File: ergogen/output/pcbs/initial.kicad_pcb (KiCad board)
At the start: 2 copper layers, 190.8 x 90.6 mm, 57 parts

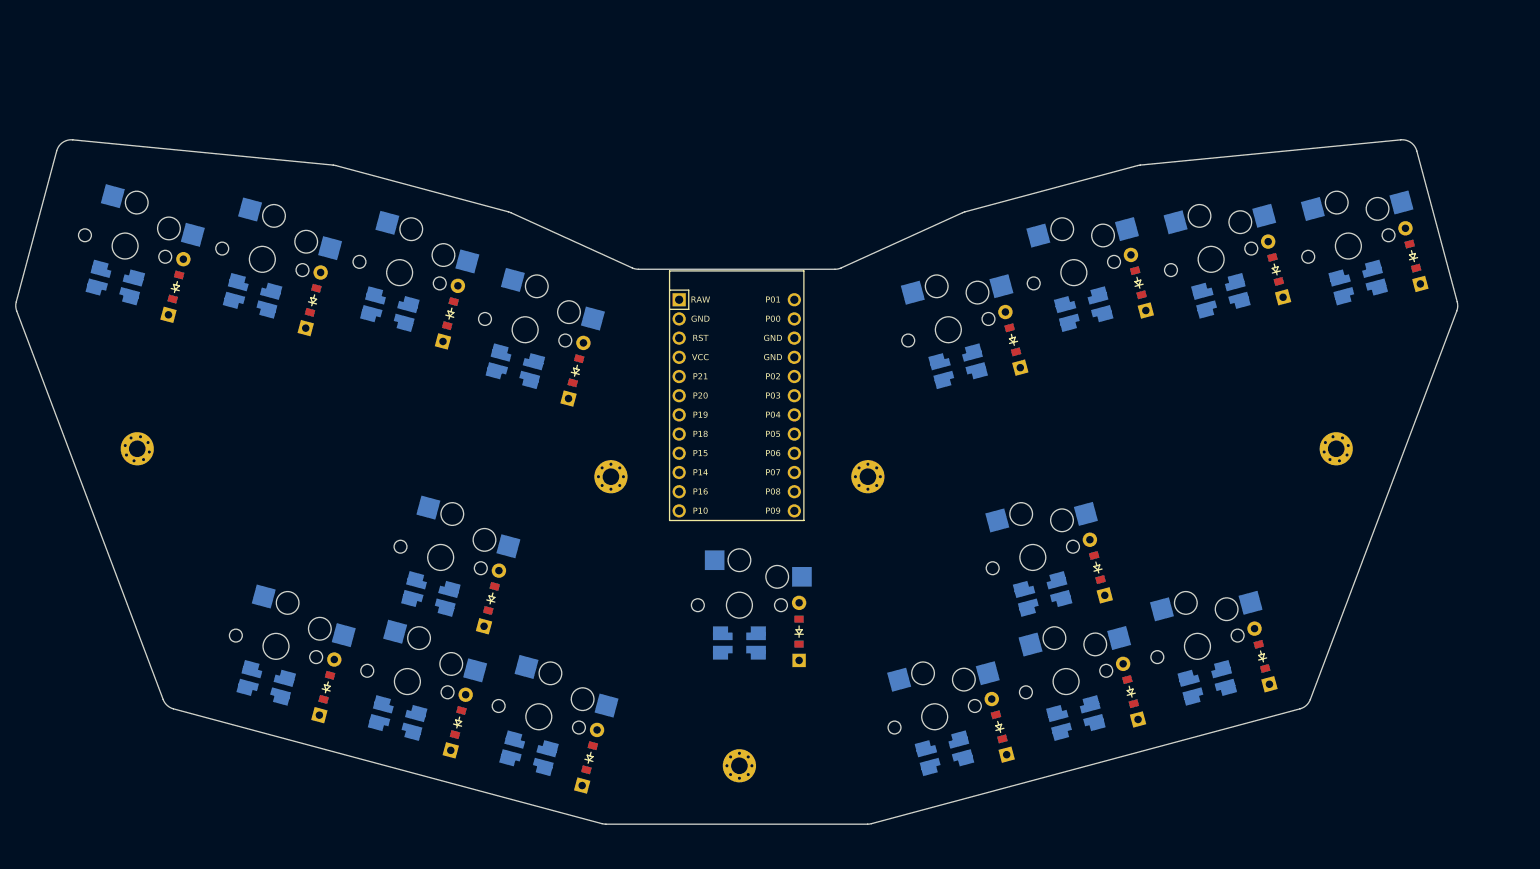
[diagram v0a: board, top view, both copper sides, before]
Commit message: yknow what eight keys
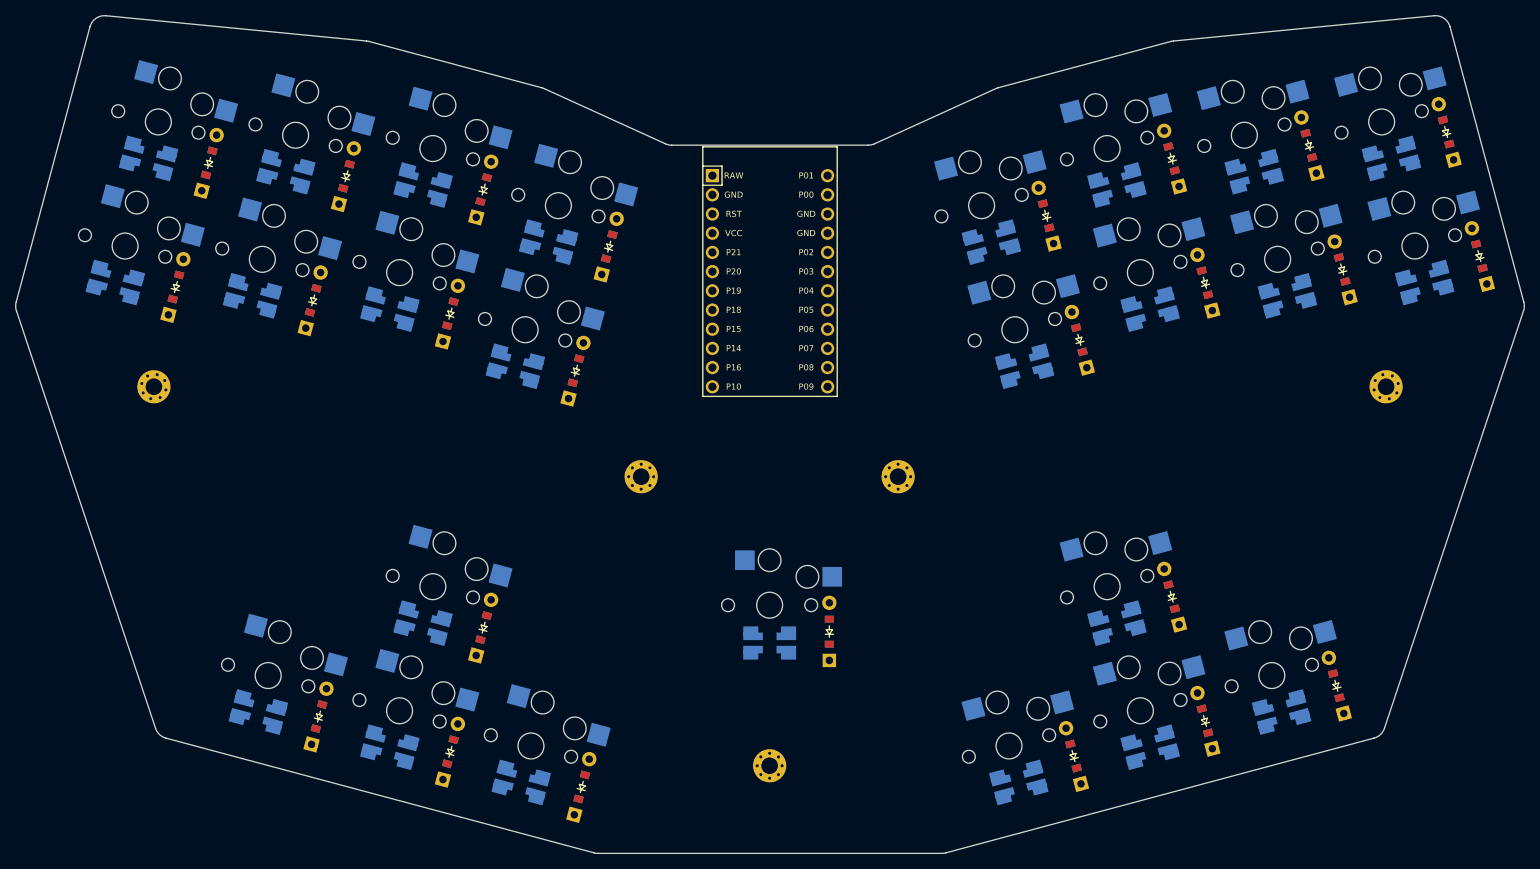
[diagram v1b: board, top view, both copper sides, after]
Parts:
- added D18: , ComboDiode, F.Cu at (213.6, 127.3)
- added D19: , ComboDiode, F.Cu at (209.2, 110.9)
- added D20: , ComboDiode, F.Cu at (197.0, 134.9)
- added D21: , ComboDiode, F.Cu at (192.6, 118.5)
- added D22: , ComboDiode, F.Cu at (231.0, 180.6)
- added D23: , ComboDiode, F.Cu at (213.6, 185.3)
- added D24: , ComboDiode, F.Cu at (209.2, 168.9)
- added D25: , ComboDiode, F.Cu at (196.2, 190.0)
- added LED18: , WS2812B, F.Cu at (206.4, 130.8)
- added LED19: , WS2812B, F.Cu at (202.0, 114.4)
- added LED20: , WS2812B, F.Cu at (189.7, 138.4)
- added LED21: , WS2812B, F.Cu at (185.3, 122.0)
- added LED22: , WS2812B, F.Cu at (223.7, 184.1)
- added LED23: , WS2812B, F.Cu at (206.4, 188.8)
- added LED24: , WS2812B, F.Cu at (202.0, 172.4)
- added LED25: , WS2812B, F.Cu at (189.0, 193.5)
- added S18: , PG1350, F.Cu at (205.1, 126.0)
- added S19: , PG1350, F.Cu at (200.7, 109.6)
- added S20: , PG1350, F.Cu at (188.4, 133.6)
- added S21: , PG1350, F.Cu at (184.0, 117.1)
- added S22: , PG1350, F.Cu at (222.4, 179.3)
- added S23: , PG1350, F.Cu at (205.1, 184.0)
- added S24: , PG1350, F.Cu at (200.7, 167.5)
- added S25: , PG1350, F.Cu at (187.7, 188.6)
- moved D10 143.3 mm to (113.8, 189.4), turned to 75 degrees
- moved LED10 142.1 mm to (105.7, 188.8), turned to -15 degrees
- moved S10 139.8 mm to (107.0, 184.0), turned to -15 degrees
- moved D11 115.0 mm to (118.2, 173.0), turned to 75 degrees
- moved LED11 114.1 mm to (110.1, 172.4), turned to -15 degrees
- moved S11 111.7 mm to (111.4, 167.5), turned to -15 degrees
- moved D12 99.4 mm to (131.1, 194.1), turned to 75 degrees
- moved LED12 97.3 mm to (123.1, 193.5), turned to -15 degrees
- moved S12 95.3 mm to (124.4, 188.6), turned to -15 degrees
- moved D17 87.2 mm to (227.4, 109.2)
- moved S17 87.2 mm to (218.8, 107.8)
- moved LED17 87.2 mm to (220.1, 112.6)
- moved D15 85.0 mm to (245.5, 107.4)
- moved S15 85.0 mm to (237.0, 106.1)
- moved LED15 85.0 mm to (238.3, 110.9)
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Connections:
- net mirror_home_top renamed mirror_ring_bottom
- net mirror_near_thumb renamed mirror_pinky_bottom
- D1 pad 1: P16 -> P19
- D1 pad 2: pinky_home -> pinky_bottom
- D10 pad 1: P6 -> P10
- D10 pad 2: mirror_pinky_home -> home_thumb
- D11 pad 1: P6 -> P8
- D11 pad 2: mirror_ring_home -> home_top
- D12 pad 1: P6 -> P10
- D12 pad 2: mirror_middle_home -> far_thumb
- D13 pad 1: P6 -> P8
- D13 pad 2: mirror_index_home -> main_default
- D14 pad 1: P9 -> P4
- D15 pad 1: P9 -> P6
- D15 pad 2: mirror_home_thumb -> mirror_pinky_home
- D16 pad 1: P8 -> P4
- D17 pad 1: P9 -> P6
- D17 pad 2: mirror_far_thumb -> mirror_ring_home
- D2 pad 2: ring_home -> pinky_home
- D3 pad 1: P16 -> P19
- D3 pad 2: middle_home -> ring_bottom
- D4 pad 2: index_home -> ring_home
- D5 pad 1: P10 -> P19
- D5 pad 2: near_thumb -> middle_bottom
- D6 pad 1: P10 -> P16
- D6 pad 2: home_thumb -> middle_home
- D7 pad 1: P8 -> P19
- D7 pad 2: home_top -> index_bottom
- D8 pad 1: P10 -> P16
- D8 pad 2: far_thumb -> index_home
- D9 pad 1: P8 -> P10
- D9 pad 2: main_default -> near_thumb
- LED1 pad 2: P18 -> P14
- LED1 pad 22: P18 -> P14
- LED1 pad 4: P18 -> P14
- LED1 pad 44: P18 -> P14
- LED10 pad 2: P18 -> P14
- LED10 pad 22: P18 -> P14
- LED10 pad 4: P18 -> P14
- LED10 pad 44: P18 -> P14
- LED11 pad 2: P18 -> P14
- LED11 pad 22: P18 -> P14
- LED11 pad 4: P18 -> P14
- LED11 pad 44: P18 -> P14
- LED12 pad 2: P18 -> P14
- LED12 pad 22: P18 -> P14
- LED12 pad 4: P18 -> P14
- LED12 pad 44: P18 -> P14
- LED13 pad 2: P18 -> P14
- LED13 pad 22: P18 -> P14
- LED13 pad 4: P18 -> P14
- LED13 pad 44: P18 -> P14
- LED14 pad 2: P18 -> P14
- LED14 pad 22: P18 -> P14
- LED14 pad 4: P18 -> P14
- LED14 pad 44: P18 -> P14
- LED15 pad 2: P18 -> P14
- LED15 pad 22: P18 -> P14
- LED15 pad 4: P18 -> P14
- LED15 pad 44: P18 -> P14
- LED16 pad 2: P18 -> P14
- LED16 pad 22: P18 -> P14
- LED16 pad 4: P18 -> P14
- LED16 pad 44: P18 -> P14
- LED17 pad 2: P18 -> P14
- LED17 pad 22: P18 -> P14
- LED17 pad 4: P18 -> P14
- LED17 pad 44: P18 -> P14
- LED2 pad 2: P18 -> P14
- LED2 pad 22: P18 -> P14
- LED2 pad 4: P18 -> P14
- LED2 pad 44: P18 -> P14
- LED3 pad 2: P18 -> P14
- LED3 pad 22: P18 -> P14
- LED3 pad 4: P18 -> P14
- LED3 pad 44: P18 -> P14
- LED4 pad 2: P18 -> P14
- LED4 pad 22: P18 -> P14
- LED4 pad 4: P18 -> P14
- LED4 pad 44: P18 -> P14
- LED5 pad 2: P18 -> P14
- LED5 pad 22: P18 -> P14
- LED5 pad 4: P18 -> P14
- LED5 pad 44: P18 -> P14
- LED6 pad 2: P18 -> P14
- LED6 pad 22: P18 -> P14
- LED6 pad 4: P18 -> P14
- LED6 pad 44: P18 -> P14
- LED7 pad 2: P18 -> P14
- LED7 pad 22: P18 -> P14
- LED7 pad 4: P18 -> P14
- LED7 pad 44: P18 -> P14
- LED8 pad 2: P18 -> P14
- LED8 pad 22: P18 -> P14
- LED8 pad 4: P18 -> P14
- LED8 pad 44: P18 -> P14
- LED9 pad 2: P18 -> P14
- LED9 pad 22: P18 -> P14
- LED9 pad 4: P18 -> P14
- LED9 pad 44: P18 -> P14
- S1 pad 2: pinky_home -> pinky_bottom
- S10 pad 1: P18 -> P15
- S10 pad 2: mirror_pinky_home -> home_thumb
- S11 pad 2: mirror_ring_home -> home_top
- S12 pad 2: mirror_middle_home -> far_thumb
- S13 pad 2: mirror_index_home -> main_default
- S15 pad 1: P15 -> P18
- S15 pad 2: mirror_home_thumb -> mirror_pinky_home
- S17 pad 1: P7 -> P15
- S17 pad 2: mirror_far_thumb -> mirror_ring_home
- S2 pad 1: P15 -> P18
- S2 pad 2: ring_home -> pinky_home
- S3 pad 1: P5 -> P15
- S3 pad 2: middle_home -> ring_bottom
- S4 pad 1: P7 -> P15
- S4 pad 2: index_home -> ring_home
- S5 pad 1: P18 -> P5
- S5 pad 2: near_thumb -> middle_bottom
- S6 pad 1: P15 -> P5
- S6 pad 2: home_thumb -> middle_home
- S7 pad 1: P15 -> P7
- S7 pad 2: home_top -> index_bottom
- S8 pad 2: far_thumb -> index_home
- S9 pad 1: P7 -> P18
- S9 pad 2: main_default -> near_thumb
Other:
- board size 190.8 x 90.6 mm -> 199.6 x 110.8 mm
- net class Default removed
